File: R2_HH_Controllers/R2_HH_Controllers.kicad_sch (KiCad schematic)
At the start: 56 parts, among them IC1 E22-900M22S, J2 USB4105-GF-A, J3 S2B-PH-SM4-TB_LF__SN_, SW1 SW_Push, SW10 Reset, SW12 Boot, SW2 SW_Push, SW3 SW_Push, SW4 SW_Push, SW5 SW_Push, SW6 SW_Push, SW7 SW_Push, SW8 SW_Push, SW9 PCM12SMTR, U2 USBLC6-2SC6, U3 BQ24074RGT, U4 ESP32-S3-MINI-1, U5 AP2112K-3.3

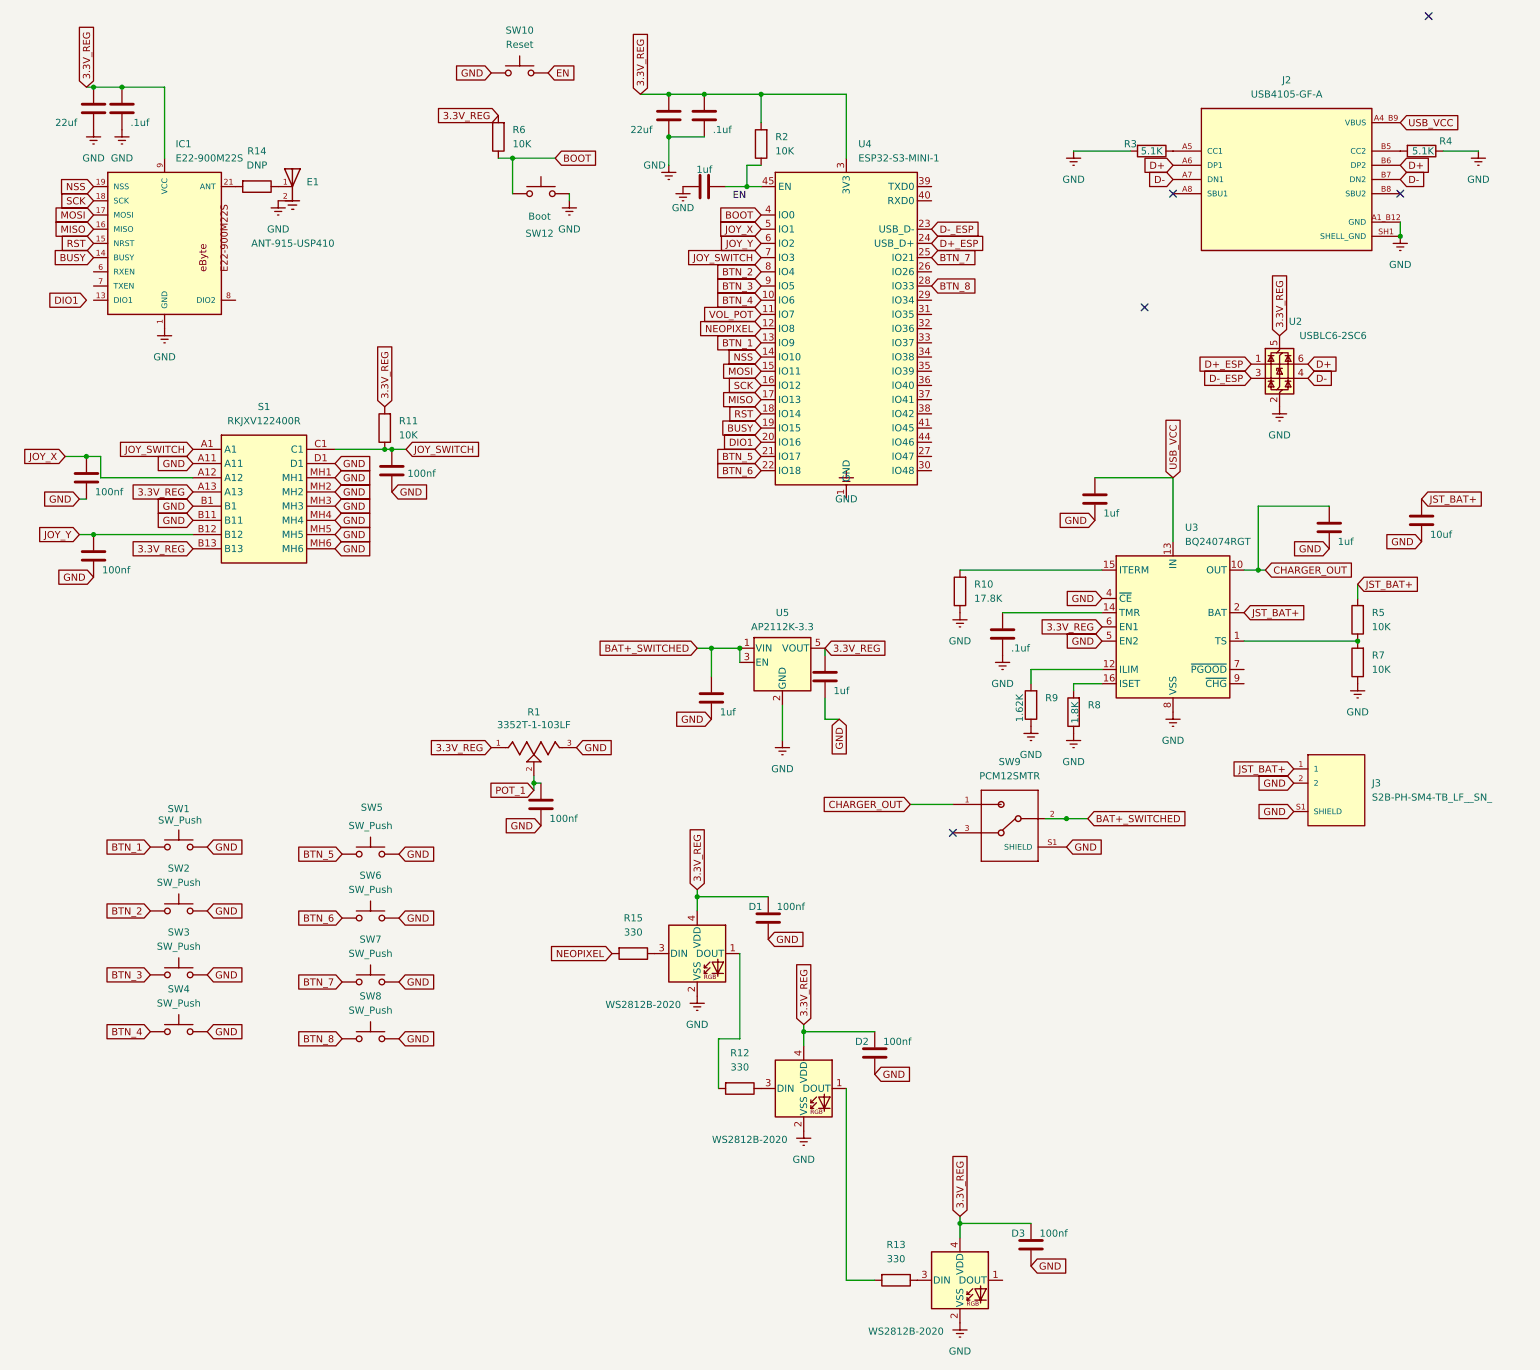
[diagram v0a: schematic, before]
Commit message: updates
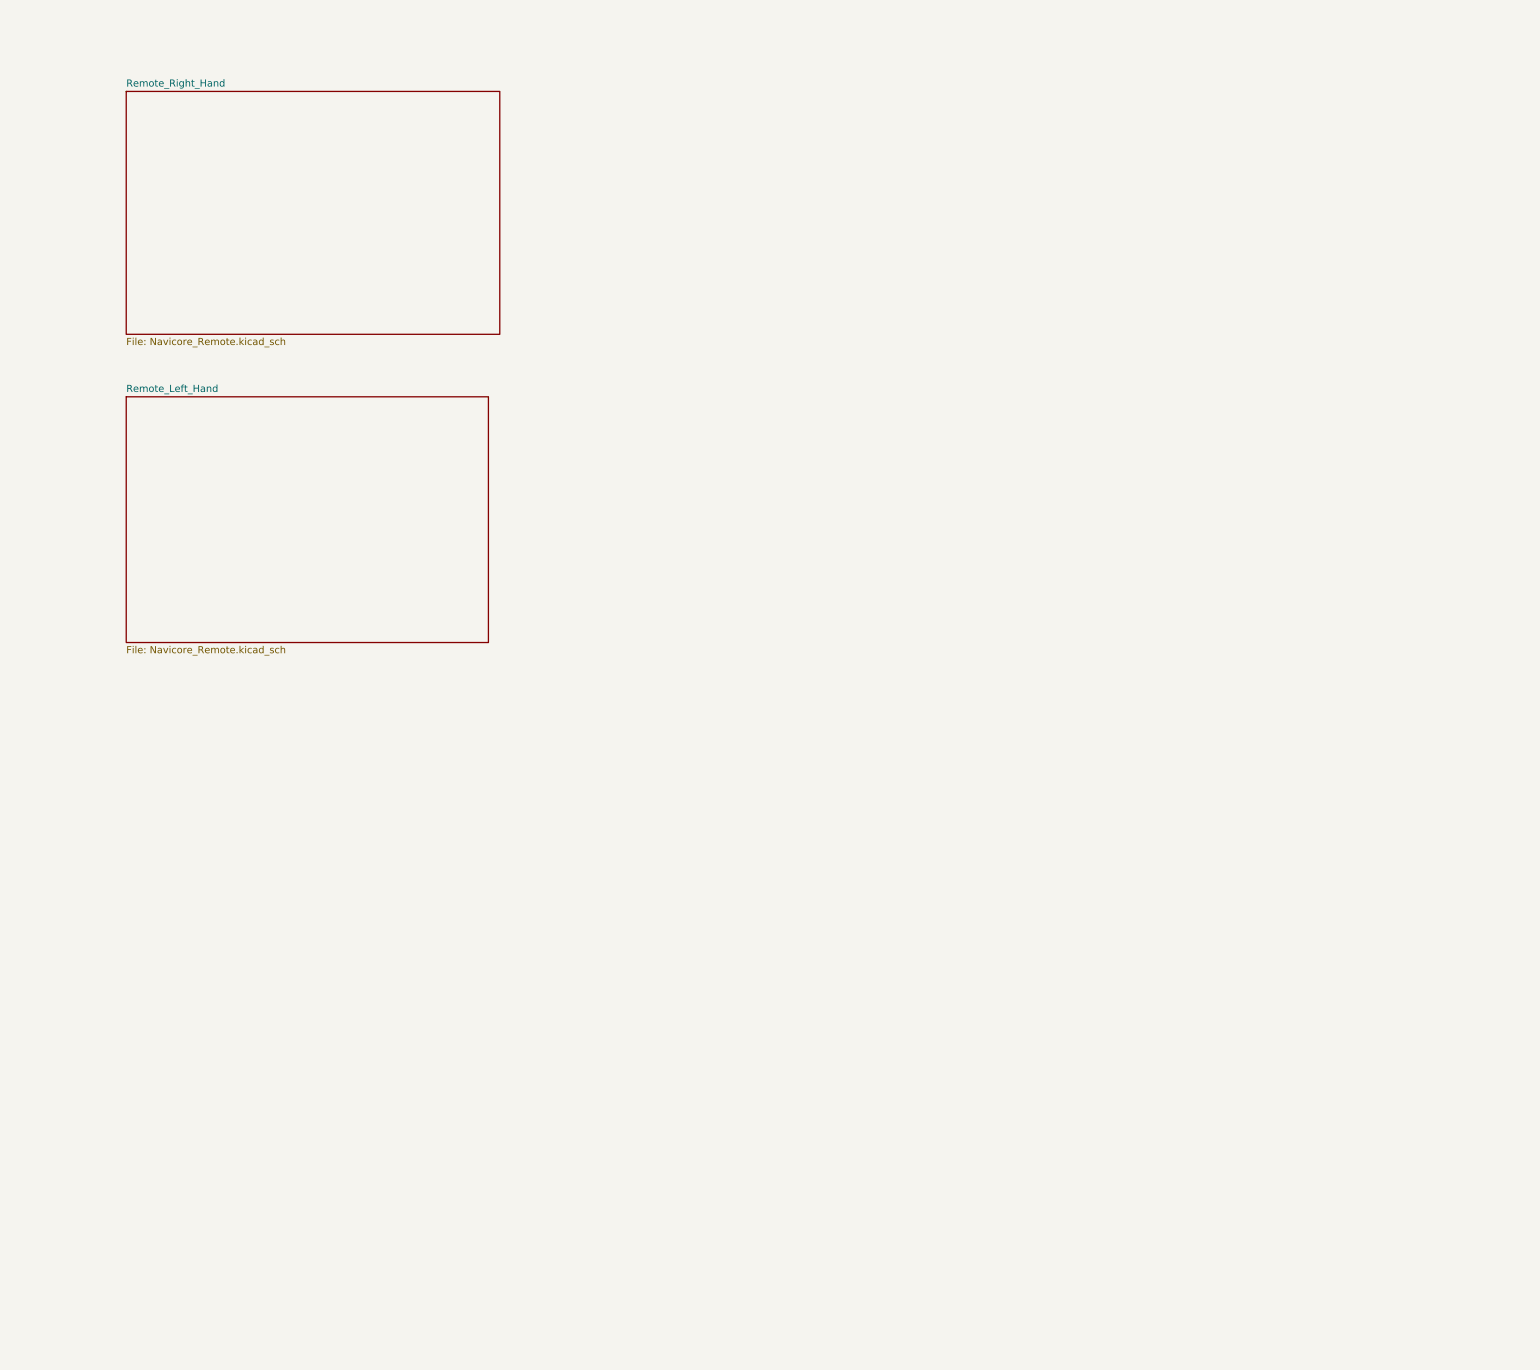
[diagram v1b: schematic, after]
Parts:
- removed C1, C5, C7, C8, C9: 1uf, Capacitor_SMD:C_0603_1608Metric, symbol Device:C
- removed C10: 22uf, Capacitor_SMD:C_0805_2012Metric_Pad1.18x1.45mm_HandSolder, symbol Device:C
- removed C11: .1uf, Capacitor_SMD:C_0805_2012Metric_Pad1.18x1.45mm_HandSolder, symbol Device:C
- removed C12, C13, C14, C15, C16, C17, C18: 100nf, Capacitor_SMD:C_0603_1608Metric, symbol Device:C
- removed C2: 22uf, Capacitor_SMD:C_0603_1608Metric, symbol Device:C
- removed C3, C4: .1uf, Capacitor_SMD:C_0603_1608Metric, symbol Device:C
- removed C6: 10uf, Capacitor_SMD:C_0603_1608Metric, symbol Device:C
- removed D1, D2, D3: WS2812B-2020, LED_SMD:LED_WS2812B-2020_PLCC4_2.0x2.0mm, symbol LED:WS2812B-2020
- removed E1: ANT-915-USP410, custom:XDCR_ANT-915-USP410, symbol 01-Custom:ANT-915-USP410
- removed IC1: E22-900M22S, custom:E22-900M22S, symbol 01-Custom:E22-900M22S
- removed J2: USB4105-GF-A, 01-Custom:GCT_USB4105-GF-A, symbol 01-Custom:USB4105-GF-A
- removed J3: S2B-PH-SM4-TB_LF__SN_, 01-Custom:JST_S2B-PH-SM4-TB_LF__SN_, symbol 01-Custom:S2B-PH-SM4-TB_LF__SN_
- removed R1: 3352T-1-103LF, 01-Custom:TRIM_3352T-1-103LF, symbol 01-Custom:3352T-1-103LF
- removed R10: 17.8K, Resistor_SMD:R_0603_1608Metric, symbol Device:R
- removed R11, R2, R5, R6, R7: 10K, Resistor_SMD:R_0603_1608Metric, symbol Device:R
- removed R12, R13, R15: 330, Resistor_SMD:R_0603_1608Metric, symbol Device:R
- removed R14: DNP, Resistor_SMD:R_0805_2012Metric_Pad1.20x1.40mm_HandSolder, symbol Device:R
- removed R3, R4: 5.1K, Resistor_SMD:R_0603_1608Metric, symbol Device:R
- removed R8: 1.8K, Resistor_SMD:R_0603_1608Metric, symbol Device:R
- removed R9: 1.62K, Resistor_SMD:R_0603_1608Metric, symbol Device:R
- removed S1: RKJXV122400R, 01-Custom:RKJXV122400R, symbol 01-Custom:RKJXV122400R
- removed SW1, SW2, SW3, SW4, SW5, SW6, SW7, SW8: SW_Push, 01-Custom:TL3360CF185Q, symbol Switch:SW_Push
- removed SW10: Reset, Button_Switch_SMD:SW_SPST_TL3342, symbol Switch:SW_Push
- removed SW12: Boot, Button_Switch_SMD:SW_SPST_TL3342, symbol Switch:SW_Push
- removed SW9: PCM12SMTR, 01-Custom:SW_PCM12SMTR, symbol 01-Custom:PCM12SMTR
- removed U2: USBLC6-2SC6, Package_TO_SOT_SMD:SOT-23-6, symbol Power_Protection:USBLC6-2SC6
- removed U3: BQ24074RGT, Package_DFN_QFN:VQFN-16-1EP_3x3mm_P0.5mm_EP1.6x1.6mm, symbol Battery_Management:BQ24074RGT
- removed U4: ESP32-S3-MINI-1, RF_Module:ESP32-S2-MINI-1, symbol RF_Module:ESP32-S3-MINI-1
- removed U5: AP2112K-3.3, Package_TO_SOT_SMD:SOT-23-5, symbol Regulator_Linear:AP2112K-3.3
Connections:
- no-connect marks 5 -> 0
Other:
- added sheet Remote_Left_Hand (Navicore_Remote.kicad_sch)
- added sheet Remote_Right_Hand (Navicore_Remote.kicad_sch)
